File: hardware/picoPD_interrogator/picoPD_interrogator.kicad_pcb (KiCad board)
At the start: 4 copper layers, 81.9 x 18.8 mm, 94 parts, among them J4 Extra Pins, J5 Conn_01x04, J6 SM03B-SRSS-TB, J7 SM04B-SRSS-TB, Q1 rohm-RE1C002UN, Q2 rohm-RE1C002UN, Q3 rohm-RE1C002UN, Q4 rohm-RE1C002UN, Q5 rohm-RE1C002UN, Q6 rohm-RE1C002UN, SW1 SW_Push, SW2 SW_Push, U1 RP2350_60QFN, U10 W25Q128JVS, U2 ST-LM393QT, U7 LV2862XDDC, Y1 Crystal_GND24

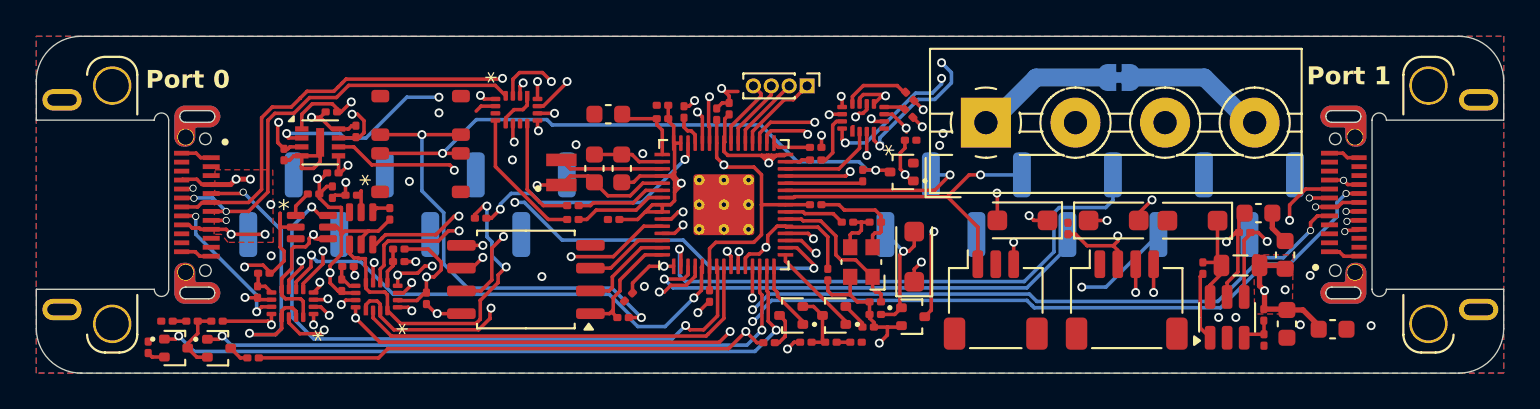
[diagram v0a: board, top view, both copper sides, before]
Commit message: PCB: Getting PCB ready for Gerber generation.
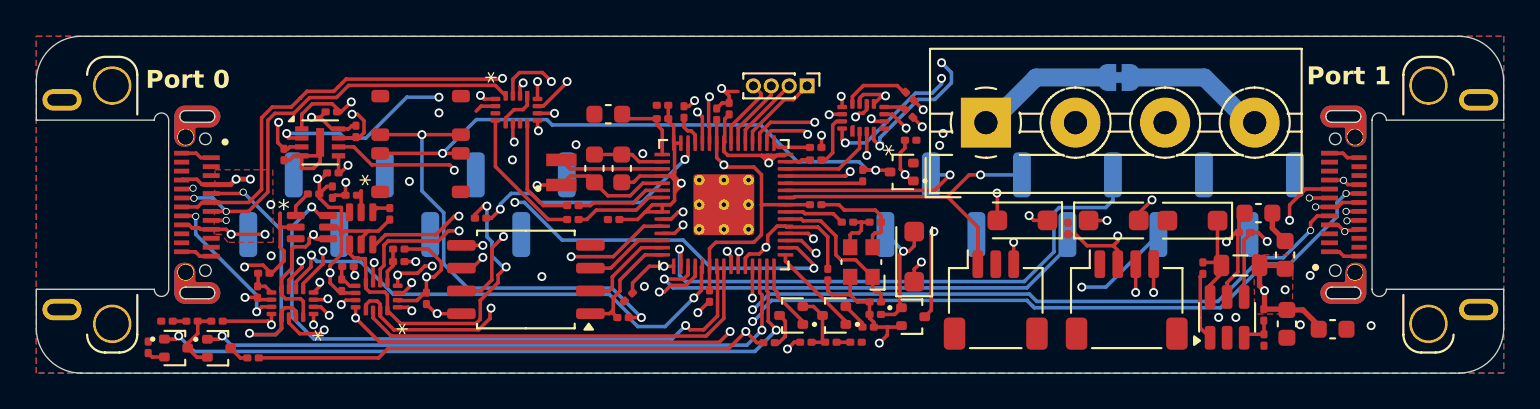
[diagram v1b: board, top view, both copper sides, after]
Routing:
- net /3V3: track 104.1 -> 105.8 mm
- net /P1_VBUS: track 19.7 -> 20.7 mm
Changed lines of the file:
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@@
 		(fp_arc
 			(start 3.521125 1.286294)
-			(mid 3.477135 1.233898)
+			(mid 3.477135 1.233899)
 			(end 3.435 1.18)
 			(stroke
@@
 		(fp_arc
 			(start 3.93363 -1.644317)
-			(mid 4.00637 -1.689264)
+			(mid 4.006369 -1.689267)
 			(end 4.081 -1.731)
 			(stroke
@@
 		(fp_arc
 			(start 5.000479 1.960685)
-			(mid 4.744554 1.943974)
+			(mid 4.744554 1.943973)
 			(end 4.493 1.894)
 			(stroke
@@
 		(fp_arc
 			(start 5.638712 -1.85392)
-			(mid 5.734863 -1.817952)
+			(mid 5.734863 -1.817951)
 			(end 5.829 -1.777)
 			(stroke
@@
 		(fp_arc
 			(start 5.829295 1.77705)
-			(mid 5.735154 1.818015)
+			(mid 5.735155 1.818016)
 			(end 5.639 1.854)
 			(stroke
@@
 		(fp_arc
 			(start 5.920652 -1.730826)
-			(mid 5.995275 -1.689024)
+			(mid 5.995274 -1.689022)
 			(end 6.068 -1.644)
 			(stroke
@@
 		(fp_arc
 			(start 6.096479 -1.625751)
-			(mid 6.166349 -1.576375)
+			(mid 6.166348 -1.576374)
 			(end 6.234 -1.524)
 			(stroke
@@
 		(fp_arc
 			(start 6.233457 1.523294)
-			(mid 6.165839 1.575648)
+			(mid 6.16584 1.575649)
 			(end 6.096 1.625)
 			(stroke
@@
 		(fp_arc
 			(start 8.521125 1.286294)
-			(mid 8.477135 1.233898)
+			(mid 8.477135 1.233899)
 			(end 8.435 1.18)
 			(stroke
@@
 		(fp_arc
 			(start 8.93363 -1.644317)
-			(mid 9.00637 -1.689264)
+			(mid 9.006369 -1.689267)
 			(end 9.081 -1.731)
 			(stroke
@@
 		(fp_arc
 			(start 10.000479 1.960685)
-			(mid 9.744554 1.943974)
+			(mid 9.744554 1.943973)
 			(end 9.493 1.894)
 			(stroke
@@
 		(fp_arc
 			(start 10.638712 -1.85392)
-			(mid 10.734863 -1.817952)
+			(mid 10.734863 -1.817951)
 			(end 10.829 -1.777)
 			(stroke
@@
 		(fp_arc
 			(start 10.829295 1.77705)
-			(mid 10.735154 1.818015)
+			(mid 10.735155 1.818016)
 			(end 10.639 1.854)
 			(stroke
@@
 		(fp_arc
 			(start 10.920652 -1.730826)
-			(mid 10.995275 -1.689024)
+			(mid 10.995274 -1.689022)
 			(end 11.068 -1.644)
 			(stroke
@@
 		(fp_arc
 			(start 11.096479 -1.625751)
-			(mid 11.166349 -1.576375)
+			(mid 11.166348 -1.576374)
 			(end 11.234 -1.524)
 			(stroke
@@
 		(fp_arc
 			(start 11.233457 1.523294)
-			(mid 11.165839 1.575648)
+			(mid 11.16584 1.575649)
 			(end 11.096 1.625)
 			(stroke
@@
 		(fp_arc
 			(start 13.521125 1.286294)
-			(mid 13.477135 1.233898)
+			(mid 13.477135 1.233899)
 			(end 13.435 1.18)
 			(stroke
@@
 		(fp_arc
 			(start 13.93363 -1.644317)
-			(mid 14.00637 -1.689264)
+			(mid 14.006369 -1.689267)
 			(end 14.081 -1.731)
 			(stroke
@@
 		(fp_arc
 			(start 15.000479 1.960685)
-			(mid 14.744554 1.943974)
+			(mid 14.744554 1.943973)
 			(end 14.493 1.894)
 			(stroke
@@
 		(fp_arc
 			(start 15.638712 -1.85392)
-			(mid 15.734863 -1.817952)
+			(mid 15.734863 -1.817951)
 			(end 15.829 -1.777)
 			(stroke
@@
 		(fp_arc
 			(start 15.829295 1.77705)
-			(mid 15.735154 1.818015)
+			(mid 15.735155 1.818016)
 			(end 15.639 1.854)
 			(stroke
@@
 		(fp_arc
 			(start 15.920652 -1.730826)
-			(mid 15.995275 -1.689024)
+			(mid 15.995274 -1.689022)
 			(end 16.068 -1.644)
 			(stroke
@@
 		(fp_arc
 			(start 16.096479 -1.625751)
-			(mid 16.166349 -1.576375)
+			(mid 16.166348 -1.576374)
 			(end 16.234 -1.524)
 			(stroke
@@
 		(fp_arc
 			(start 16.233457 1.523294)
-			(mid 16.165839 1.575648)
+			(mid 16.16584 1.575649)
 			(end 16.096 1.625)
 			(stroke
@@
 		(at 135.63 101.32 -90)
 		(property "Reference" "U4"
-			(at 0 -2.75 270)
+			(at 0 -2.75 -90)
 			(unlocked yes)
 			(layer "F.SilkS")
@@
 		(at 144.3 94.7 -90)
 		(property "Reference" "U8"
-			(at -0.62 -2.54 270)
+			(at -0.62 -2.54 -90)
 			(unlocked yes)
 			(layer "F.SilkS")
@@
 		(tags "capacitor")
 		(property "Reference" "C15"
-			(at 0 -1.05 270)
+			(at 0 -1.05 -90)
 			(layer "F.SilkS")
 			(hide yes)
@@
 	)
 	(segment
+		(start 189.675 101.125)
+		(end 190.155 101.125)
+		(width 0.2)
+		(layer "F.Cu")
+		(net 25)
+	)
+	(segment
 		(start 179.03 100.47)
 		(end 179.77 99.73)
@@
 		(net 25)
 	)
+	(segment
+		(start 190.155 101.125)
+		(end 190.53 101.5)
+		(width 0.2)
+		(layer "F.Cu")
+		(net 25)
+	)
 	(via
 		(at 190.46 98.64)
@@
 	)
 	(segment
+		(start 129.83 105.175)
+		(end 129.85 105.195)
+		(width 0.2)
+		(layer "F.Cu")
+		(net 31)
+	)
+	(segment
 		(start 159.3125 101.2)
 		(end 158.84935 101.2)
@@
 	)
 	(segment
-		(start 129.955 105.3)
-		(end 130.625 105.3)
-		(width 0.2)
-		(layer "F.Cu")
-		(net 31)
-	)
-	(segment
-		(start 129.85 105.195)
-		(end 129.17 105.195)
-		(width 0.2)
-		(layer "F.Cu")
-		(net 31)
-	)
-	(segment
 		(start 161.675 101.794974)
 		(end 161.675 103.58)
@@
 	)
 	(segment
+		(start 129.955 105.3)
+		(end 129.85 105.195)
+		(width 0.2)
+		(layer "F.Cu")
+		(net 31)
+	)
+	(segment
 		(start 177.86 103.32)
 		(end 177.86 102.545001)
@@
 	)
 	(segment
-		(start 129.85 105.195)
+		(start 130.625 105.3)
 		(end 129.955 105.3)
 		(width 0.2)
@@
 	)
 	(segment
+		(start 129.15 105.175)
+		(end 129.83 105.175)
+		(width 0.2)
+		(layer "F.Cu")
+		(net 31)
+	)
+	(segment
 		(start 157.075 102.97435)
 		(end 157.075 103.4375)
@@
 	)
 	(segment
+		(start 156.07 105.94)
+		(end 156.15 106.02)
+		(width 0.2)
+		(layer "In2.Cu")
+		(net 31)
+	)
+	(segment
+		(start 157.1 107.075)
+		(end 157.1 106.97)
+		(width 0.2)
+		(layer "In2.Cu")
+		(net 31)
+	)
+	(segment
+		(start 157.1 106.97)
+		(end 156.07 105.94)
+		(width 0.2)
+		(layer "In2.Cu")
+		(net 31)
+	)
+	(segment
 		(start 169.560661 98.335)
 		(end 170.2 98.335)
@@
 	)
 	(segment
+		(start 191.325 100.875)
+		(end 190.675 100.875)
+		(width 0.2)
+		(layer "F.Cu")
+		(net 55)
+	)
+	(segment
 		(start 190.705 100.875)
 		(end 190.65 100.93)
@@
 	)
 	(segment
-		(start 166.475 94.175)
-		(end 167 94.7)
+		(start 190.675 100.875)
+		(end 190.65 100.9)
 		(width 0.2)
 		(layer "F.Cu")
@@
 	)
 	(segment
-		(start 191.325 100.875)
-		(end 190.705 100.875)
+		(start 166.475 94.175)
+		(end 167 94.7)
 		(width 0.2)
 		(layer "F.Cu")
@@
 	)
 	(via
-		(at 190.65 100.93)
+		(at 190.65 100.9)
 		(size 0.4)
 		(drill 0.3)
@@
 	)
 	(segment
+		(start 190.625 100.875)
+		(end 190.65 100.9)
+		(width 0.2)
+		(layer "In1.Cu")
+		(net 55)
+	)
+	(segment
 		(start 188.158513 94.123461)
 		(end 188.158513 98.575)
@@
 	(segment
 		(start 188.55 100.875)
-		(end 190.595 100.875)
+		(end 190.625 100.875)
 		(width 0.2)
 		(layer "In1.Cu")
@@
 			(pts
 				(xy 127.465 98.05) (xy 130.69 98.05) (xy 130.715 102.1) (xy 132.12 106.38) (xy 155.7 106.71) (xy 156.01 107.46)
-				(xy 157.95 107.46) (xy 158.33 106.74) (xy 168.53 106.75) (xy 168.56 93.5) (xy 172.52 93.52) (xy 172.49 108.92)
+				(xy 157.95 107.46) (xy 158.33 106.74) (xy 168.79 106.75) (xy 168.78 93.65) (xy 172.52 93.52) (xy 172.49 108.92)
 				(xy 129.79 108.88) (xy 128.81 104.84) (xy 127.325 101.7)
 			)
